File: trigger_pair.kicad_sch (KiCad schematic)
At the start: 51 parts, among them J4 AudioJack2, J5 AudioJack2, J8 Conn_01x02_Pin, J9 Conn_01x02_Pin, U1 1SS362FV_L3F, U2 1SS362FV_L3F, U3 LM2902PWR, U4 1SS362FV_L3F, U5 1SS362FV_L3F, U6 1SS362FV_L3F, U7 1SS362FV_L3F

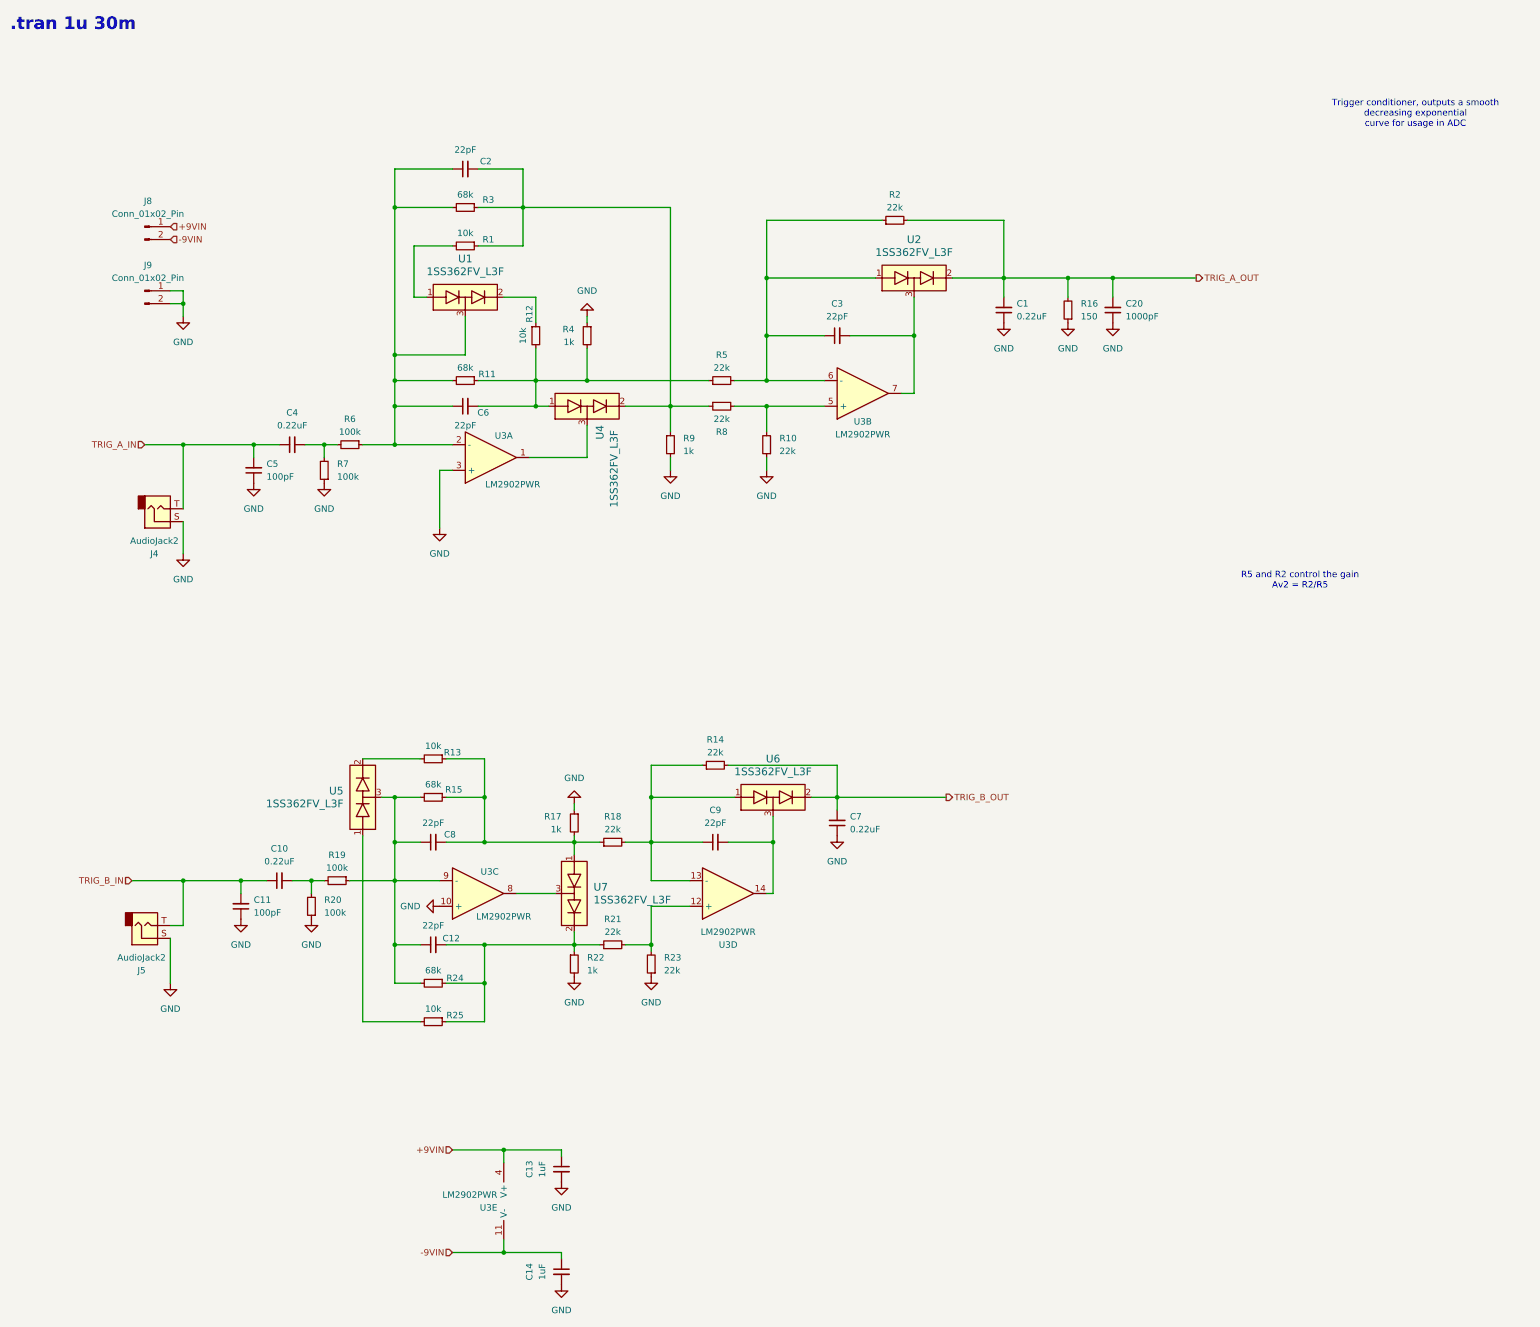
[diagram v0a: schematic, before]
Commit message: Initial layout
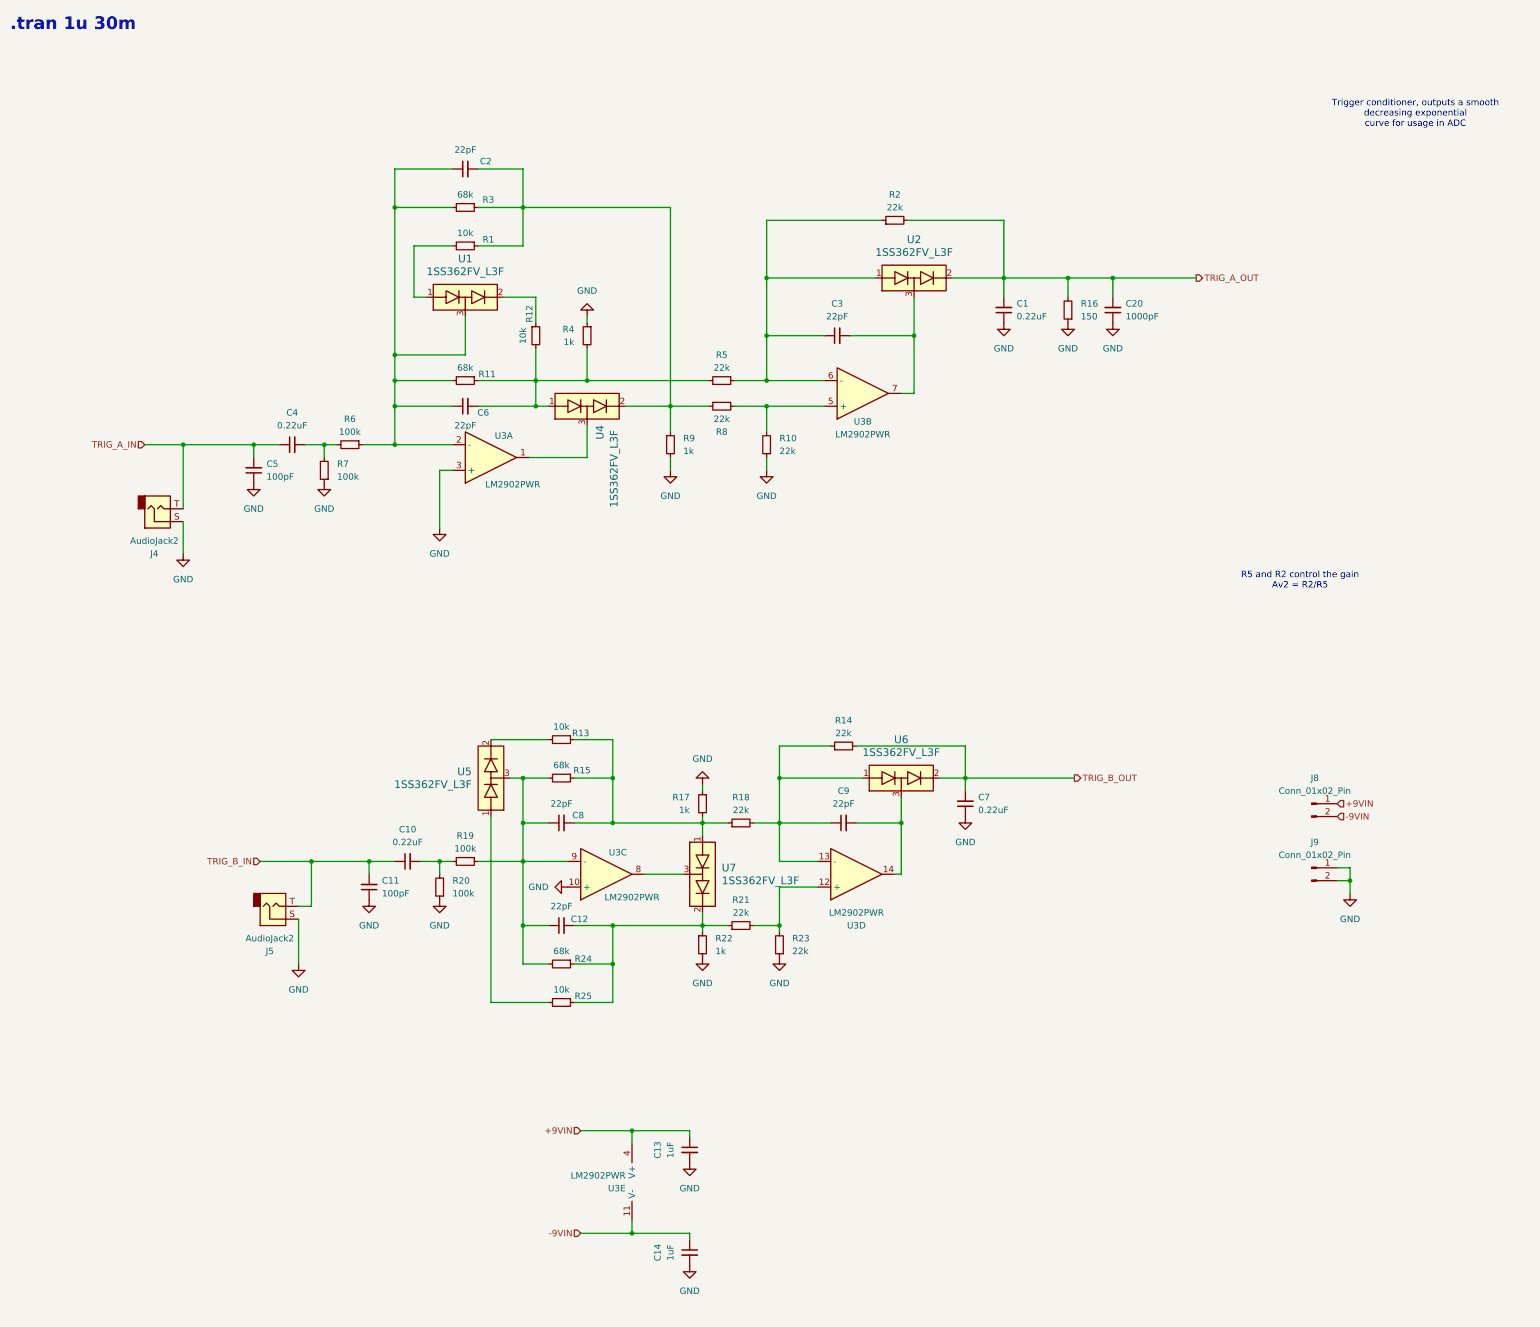
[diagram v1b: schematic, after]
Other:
- moved on the sheet: C10, C11, C12, C13, C14, C7, C8, C9, J5, J8, J9, R13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
